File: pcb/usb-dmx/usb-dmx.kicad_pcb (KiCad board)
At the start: 2 copper layers, 25 x 40 mm, 17 parts, among them J1 USB_C_Receptacle_USB2.0_16P, J2 USB_A, SW1 PTS526_SM15_SMTR2_LFS, U1 ESP32-S3-MINI-1U, U2 IP4234CZ6, U3 ADP2108AUJ-3.3, U4 ST485E

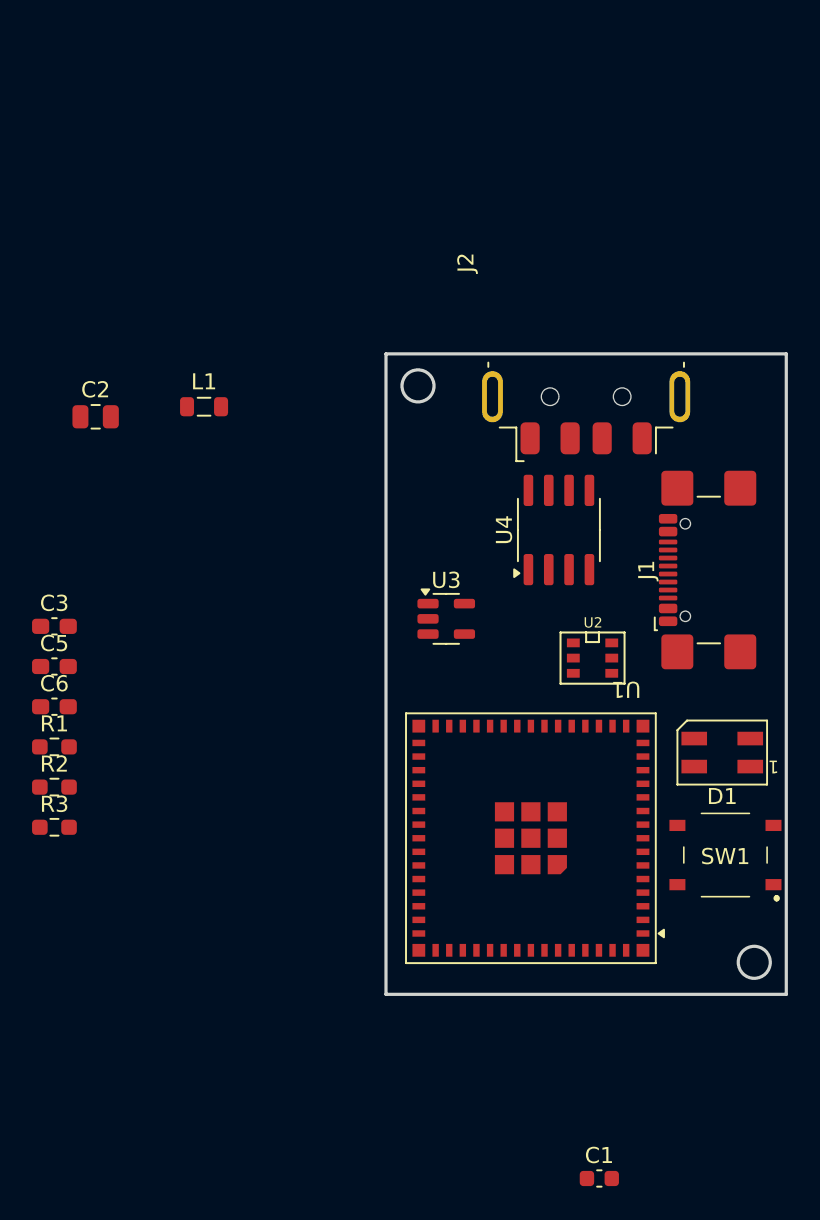
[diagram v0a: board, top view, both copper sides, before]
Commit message: creating pcb for usb-dmx
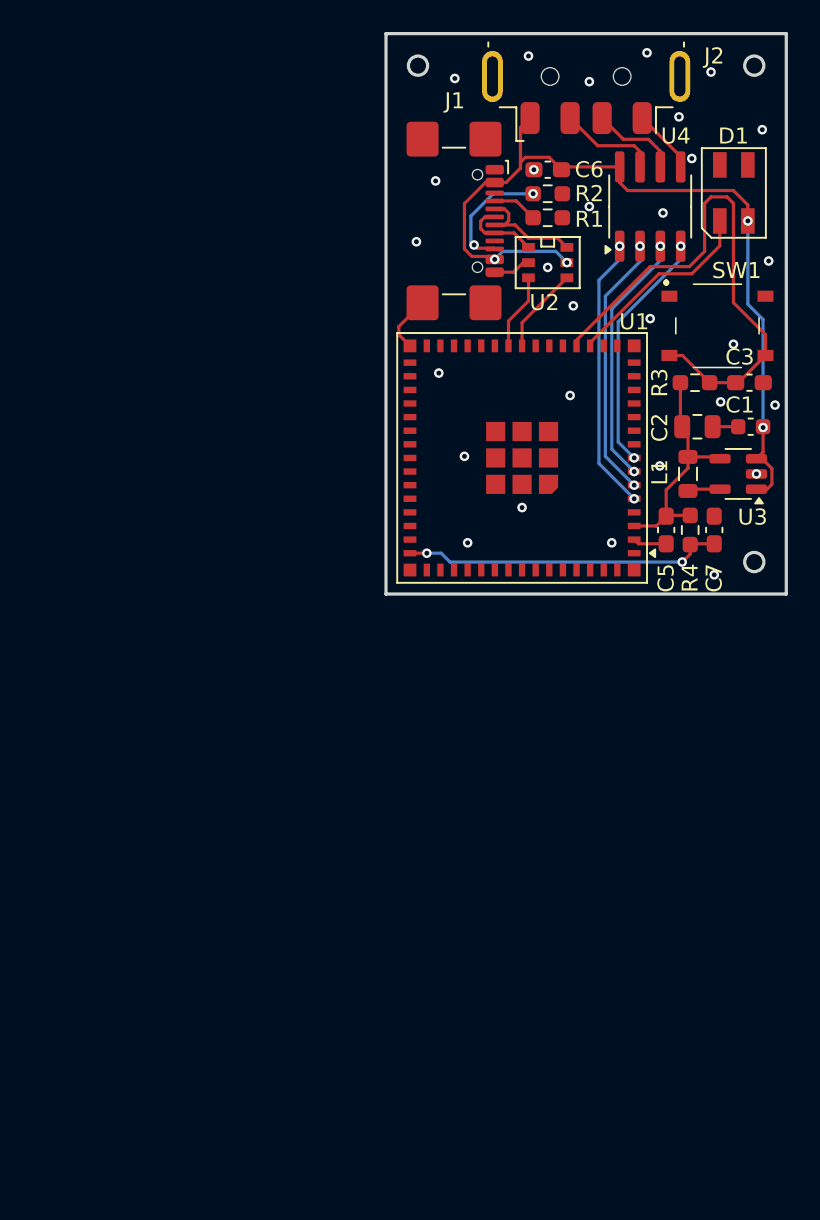
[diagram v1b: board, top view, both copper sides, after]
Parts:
- added C7: 1uF, Capacitor_SMD:C_0603_1608Metric_Pad1.08x0.95mm_HandSolder, F.Cu at (108.0, 91.0)
- added R4: 10k, Resistor_SMD:R_0603_1608Metric_Pad0.98x0.95mm_HandSolder, F.Cu at (106.5, 91.0)
- J1: value USB_C_Receptacle_USB2.0_16P -> USB_C
- moved R3 48.7 mm to (106.8, 81.8)
- moved R2 48.2 mm to (97.6, 70.0)
- moved C1 47.9 mm to (110.3, 84.5), turned to 180 degrees
- moved C3 46.0 mm to (110.2, 81.8)
- moved C6 45.5 mm to (97.6, 68.5), turned to 180 degrees
- moved R1 45.2 mm to (97.6, 71.5)
- moved C5 39.1 mm to (105.0, 91.0), turned to -90 degrees
- moved C2 37.6 mm to (107.0, 84.5)
- moved D1 35.0 mm to (109.2, 70.0), turned to -90 degrees
- moved SW1 33.1 mm to (108.2, 78.2), turned to 0 degrees
- moved L1 30.5 mm to (106.4, 87.5), turned to 90 degrees
- moved J1 28.4 mm to (90.6, 71.7), turned to -90 degrees
- moved U2 24.9 mm to (97.6, 74.3)
- moved U1 23.8 mm to (96.0, 86.5)
- moved U4 21.0 mm to (104.0, 70.8)
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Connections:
- U1 pad 45: unconnected-(U1-EN-Pad45) -> Net-(U1-EN)
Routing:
- net VCC_5V: track 0.00 -> 54.2 mm, vias 0 -> 4
- net 15: track 0.00 -> 33.5 mm
- net Net-(U1-EN): track 0.00 -> 20.0 mm, vias 0 -> 2
- net 1: track 0.00 -> 17.2 mm, vias 0 -> 2
- net 2: track 0.00 -> 16.6 mm, vias 0 -> 2
- net 3: track 0.00 -> 15.9 mm, vias 0 -> 2
- net 4: track 0.00 -> 15.3 mm, vias 0 -> 2
- net VCC_3.3V: track 0.00 -> 14.9 mm
- net GND: track 0.00 -> 13.7 mm, vias 0 -> 29
- net 14: track 0.00 -> 12.4 mm
- net Net-(J1-CC2): track 0.00 -> 7.74 mm, vias 0 -> 2
- net Net-(J1-D--PadA7): track 0.00 -> 7.53 mm
- net DMX-: track 0.00 -> 6.19 mm
- net DMX+: track 0.00 -> 5.47 mm
- net D-: track 0.00 -> 5.41 mm
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- added copper zone on B.Cu, net GND
- added copper zone on F.Cu, net GND
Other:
- board size 25 x 40 mm -> 25 x 35 mm
